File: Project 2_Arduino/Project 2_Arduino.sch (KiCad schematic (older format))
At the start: 28 parts, among them J3 USB_microB_2040002-1, J4 Conn_02x03_Odd_Even, SW1 SW_Push, U1 FT232RL, U3 ATMEGA328P-AU, Y1 16MHz

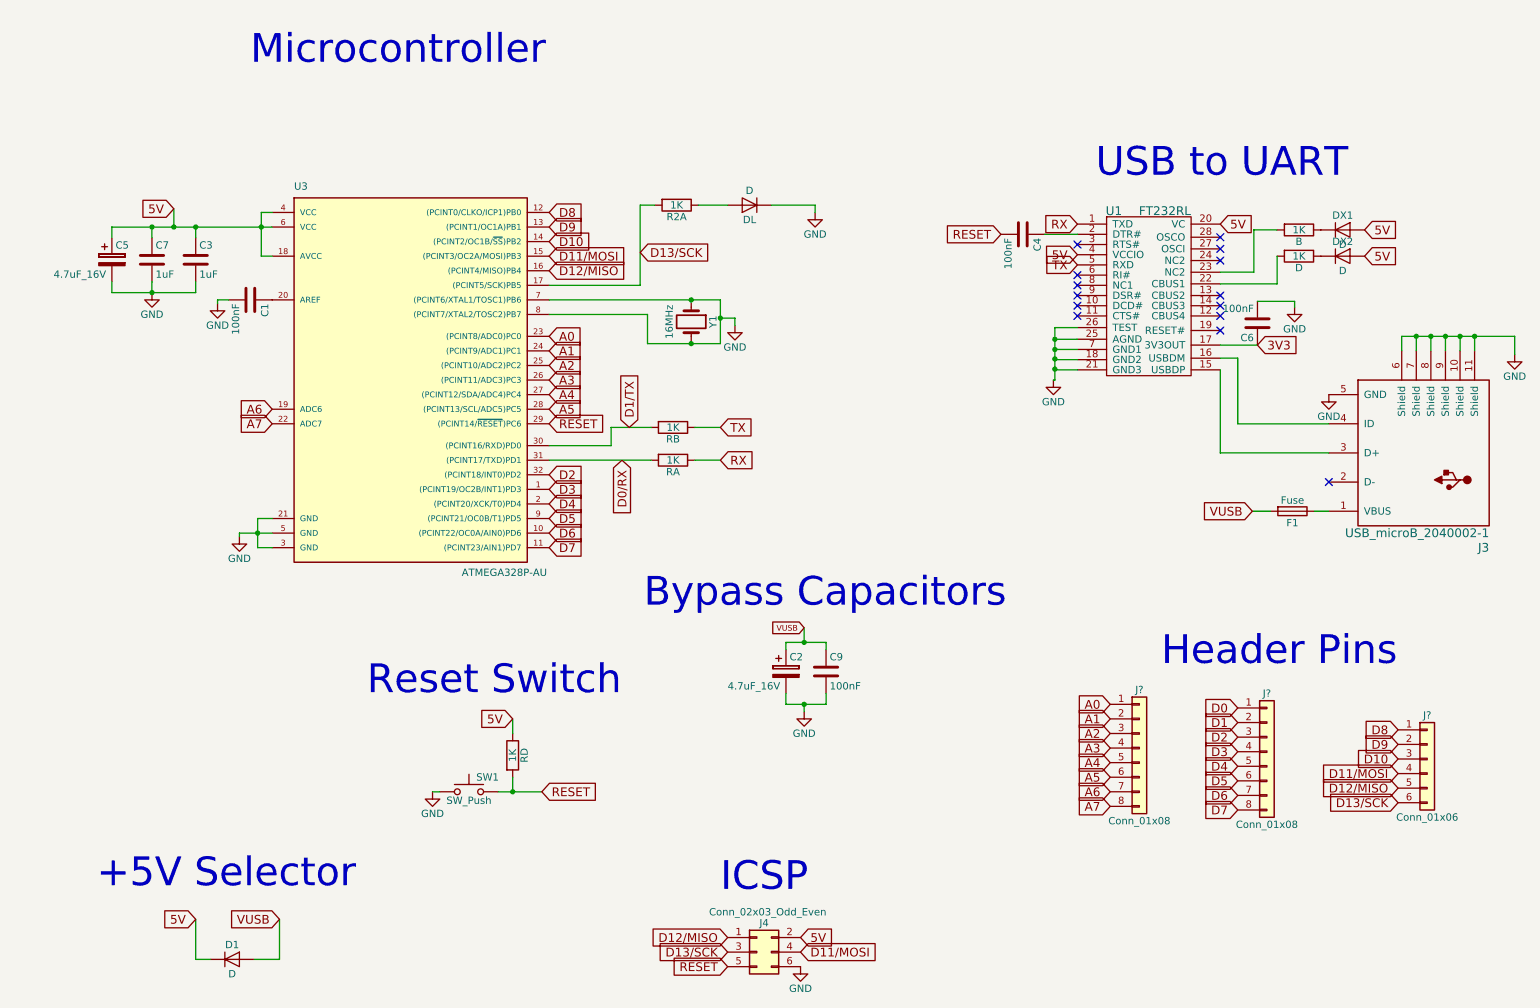
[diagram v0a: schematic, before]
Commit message: rearrange
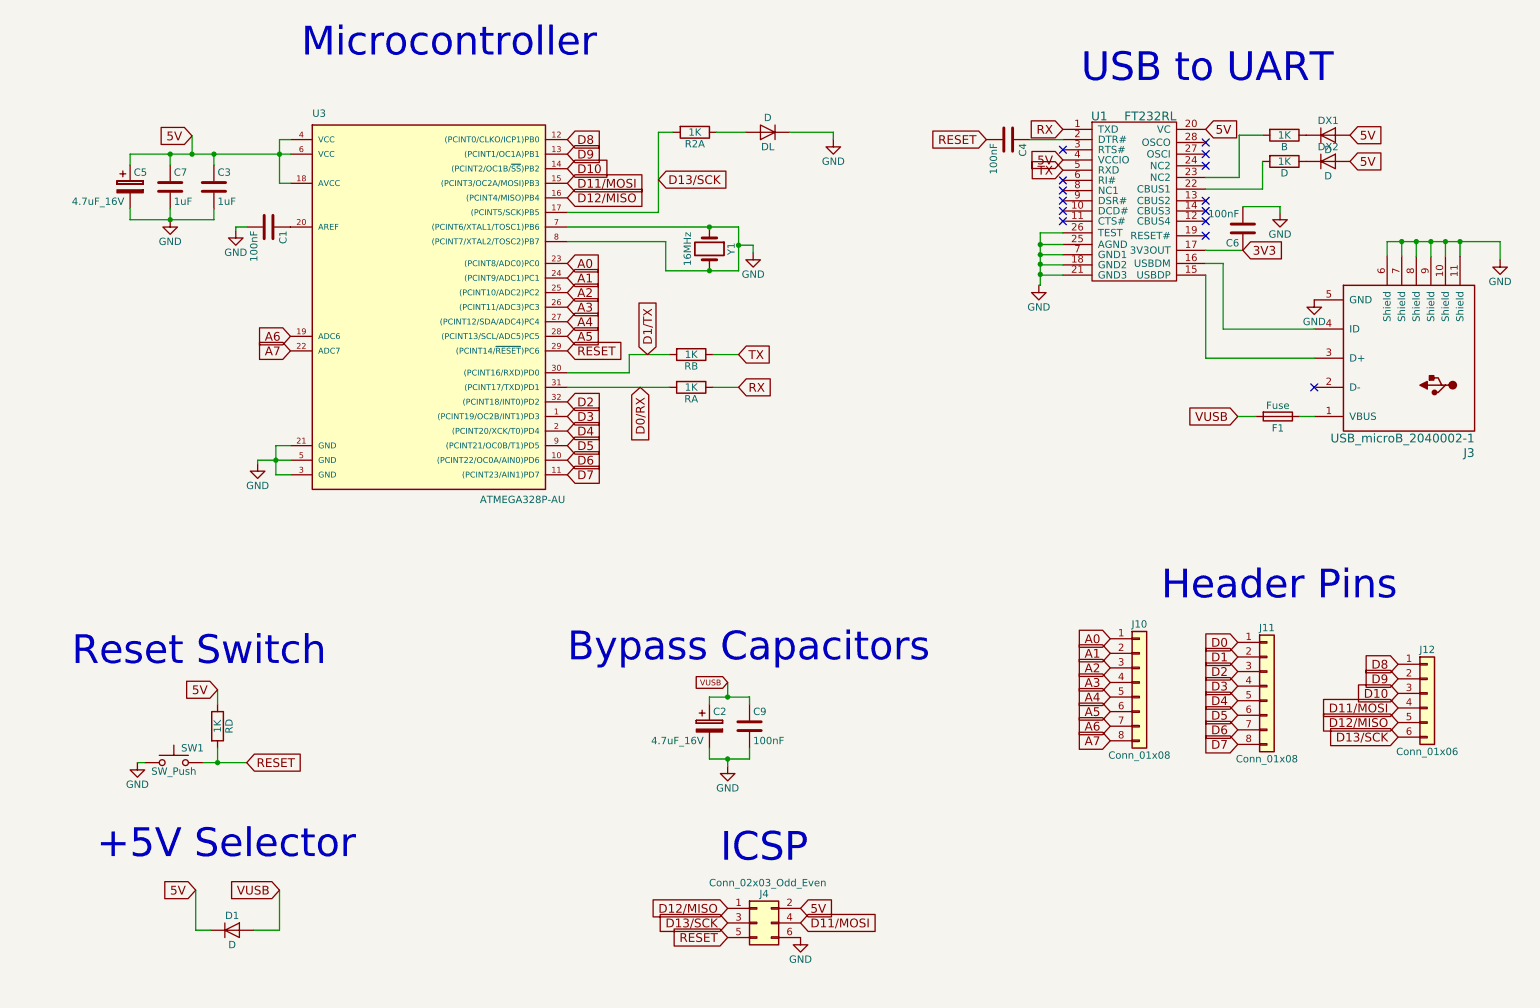
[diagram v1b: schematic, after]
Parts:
- gave numbers to parts that had none: 3
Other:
- moved on the sheet: B, C1, C2, C3, C4, C5, C6, C7, C9, D, D1, DL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
